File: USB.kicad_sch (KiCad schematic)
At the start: 15 parts, among them J2 USB4215-03-A, U8 CP2102N-A02-GQFN24

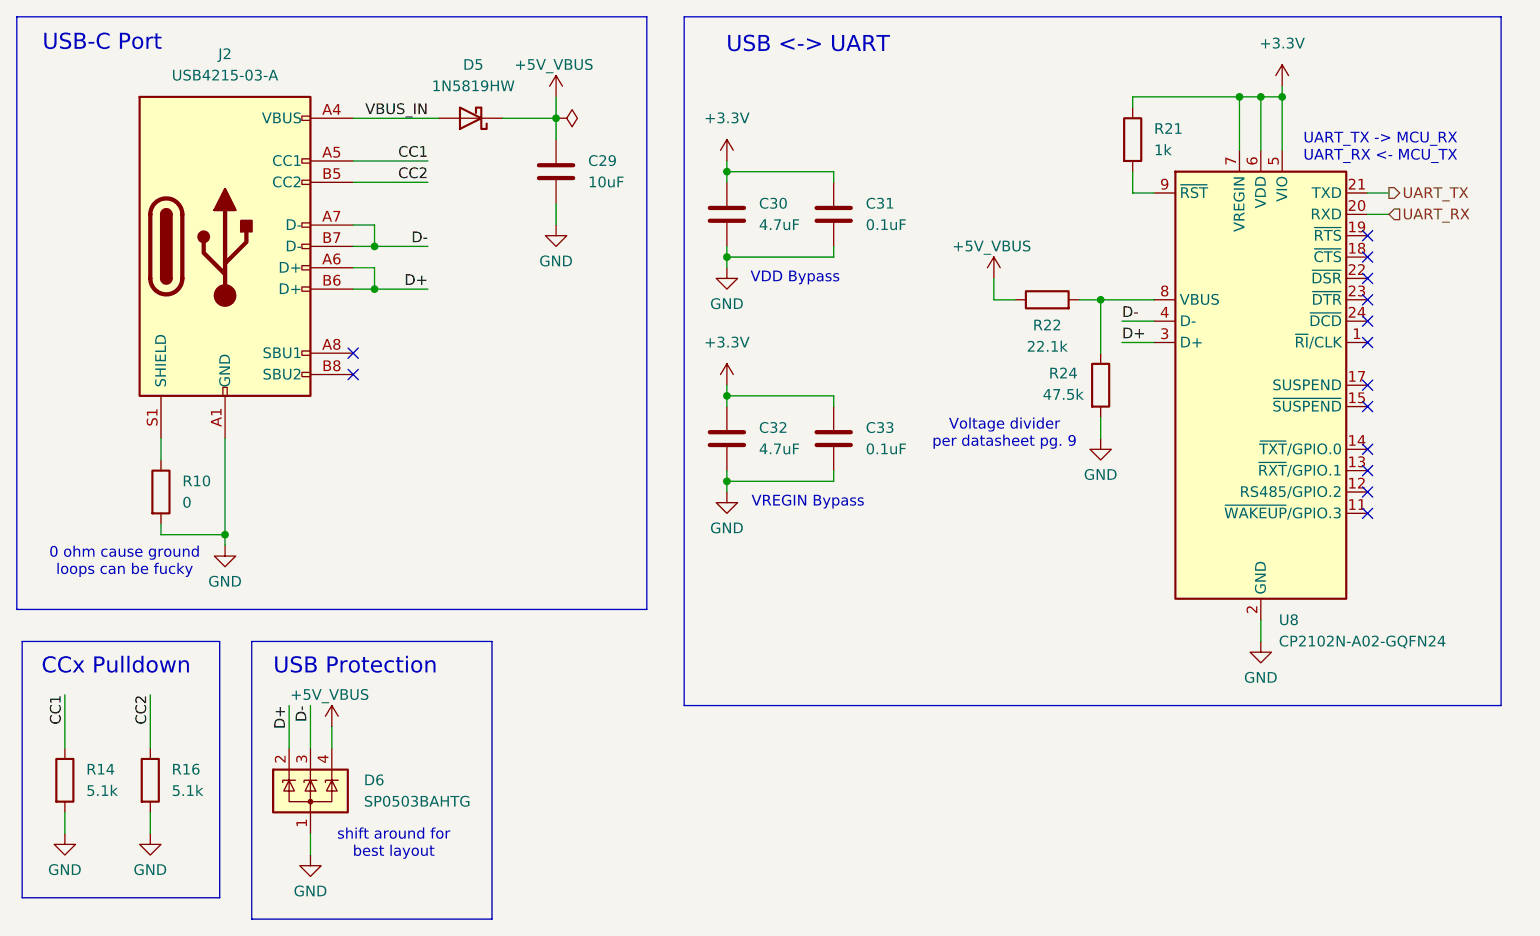
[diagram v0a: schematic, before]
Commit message: finish mcu breakouts
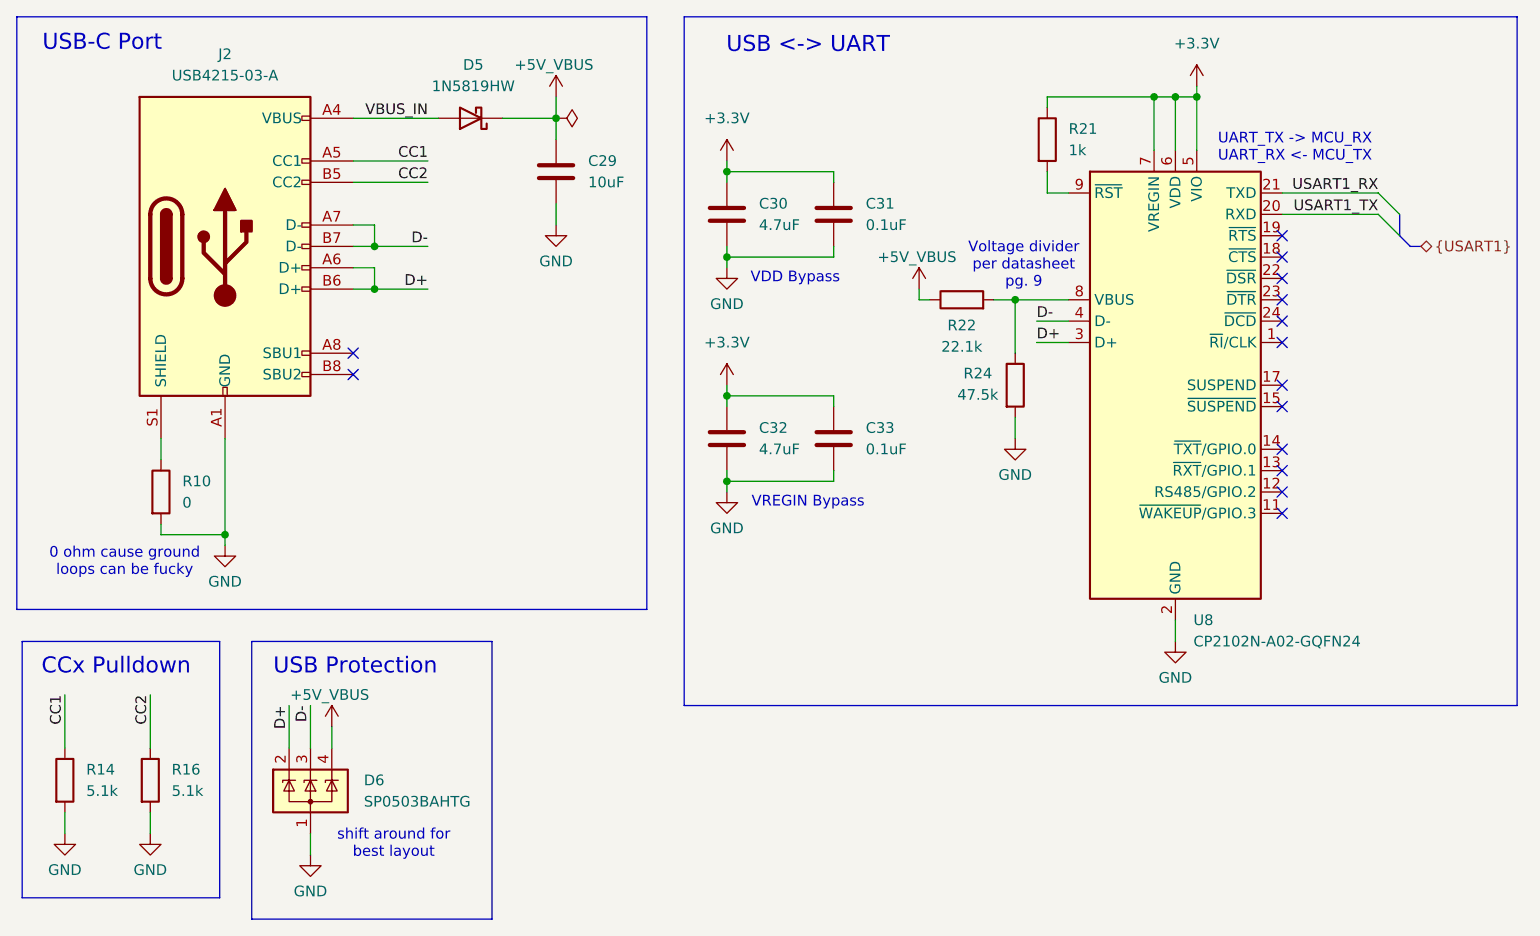
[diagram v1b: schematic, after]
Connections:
- net UART_RX renamed USART1_TX
- net UART_TX renamed USART1_RX
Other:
- moved on the sheet: R21, R22, R24, U8

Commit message: FUCK capacitors
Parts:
- C29: P/N (none) -> GRM21BR61H106KE43K
- C30, C32: P/N (none) -> 08055D475KAT4A
- C31, C33: P/N (none) -> MLASH168SB7104KTNA01
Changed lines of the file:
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@@
+			)
+		)
+		(property "P/N" "08055D475KAT4A"
+			(at 100.33 39.37 0)
+			(effects
+				(font
+					(size 1.27 1.27)
+				)
+				(hide yes)
 			)
 		)
@@
 			)
 		)
+		(property "P/N" "MLASH168SB7104KTNA01"
+			(at 113.03 66.04 0)
+			(effects
+				(font
+					(size 1.27 1.27)
+				)
+				(hide yes)
+			)
+		)
 		(pin "1"
 		)
@@
 			)
 		)
+		(property "P/N" "08055D475KAT4A"
+			(at 100.33 66.04 0)
+			(effects
+				(font
+					(size 1.27 1.27)
+				)
+				(hide yes)
+			)
+		)
 		(pin "1"
 		)
@@
 			)
 		)
+		(property "P/N" "MLASH168SB7104KTNA01"
+			(at 113.03 39.37 0)
+			(effects
+				(font
+					(size 1.27 1.27)
+				)
+				(hide yes)
+			)
+		)
 		(pin "1"
 		)
@@
 			(at 80.01 34.29 0)
 			(effects
+				(font
+					(size 1.27 1.27)
+				)
+				(hide yes)
+			)
+		)
+		(property "P/N" "GRM21BR61H106KE43K"
+			(at 80.01 34.29 0)
+			(effects

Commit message: all parts selected
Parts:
- R10: P/N (none) -> CRCW06030000Z0EI
- R14, R16: P/N (none) -> CRCW06035K10FKEC
- R21: P/N (none) -> CRCW06031K00FKEI
- R22: P/N (none) -> CRCW060322K1FKEBC
- R24: P/N (none) -> CRCW060347K5FKEAHP
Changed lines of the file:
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@@
+			)
+		)
+		(property "P/N" "CRCW06030000Z0EI "
+			(at 33.02 72.39 0)
+			(effects
+				(font
+					(size 1.27 1.27)
+				)
+				(hide yes)
 			)
 		)
@@
 		)
 		(property "Description" "Resistor"
+			(at 134.62 59.69 0)
+			(effects
+				(font
+					(size 1.27 1.27)
+				)
+				(hide yes)
+			)
+		)
+		(property "P/N" "CRCW060347K5FKEAHP "
 			(at 134.62 59.69 0)
 			(effects
@@
 			)
 		)
+		(property "P/N" "CRCW06035K10FKEC "
+			(at 31.75 106.68 0)
+			(effects
+				(font
+					(size 1.27 1.27)
+				)
+				(hide yes)
+			)
+		)
 		(pin "1"
 		)
@@
 		(property "Description" "Resistor"
 			(at 128.27 49.53 0)
+			(effects
+				(font
+					(size 1.27 1.27)
+				)
+				(hide yes)
+			)
+		)
+		(property "P/N" "CRCW060322K1FKEBC "
+			(at 128.27 49.53 90)
 			(effects
 				(font
@@
 			)
 		)
+		(property "P/N" "CRCW06031K00FKEI "
+			(at 138.43 30.48 0)
+			(effects
+				(font
+					(size 1.27 1.27)
+				)
+				(hide yes)
+			)
+		)
 		(pin "1"
 		)
@@
 			(at 21.59 106.68 0)
 			(effects
+				(font
+					(size 1.27 1.27)
+				)
+				(hide yes)
+			)
+		)
+		(property "P/N" "CRCW06035K10FKEC "
+			(at 21.59 106.68 0)
+			(effects

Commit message: add some footprints
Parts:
- R10, R14, R16, R21, R22, R24: footprint (none) -> Resistor_SMD:R_0603_1608Metric_Pad0.98x0.95mm_HandSolder
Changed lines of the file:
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@@
 			)
 		)
-		(property "Footprint" ""
+		(property "Footprint" "Resistor_SMD:R_0603_1608Metric_Pad0.98x0.95mm_HandSolder"
 			(at 31.242 72.39 90)
 			(effects
@@
 			)
 		)
-		(property "Footprint" ""
+		(property "Footprint" "Resistor_SMD:R_0603_1608Metric_Pad0.98x0.95mm_HandSolder"
 			(at 132.842 59.69 90)
 			(effects
@@
 			)
 		)
-		(property "Footprint" ""
+		(property "Footprint" "Resistor_SMD:R_0603_1608Metric_Pad0.98x0.95mm_HandSolder"
 			(at 29.972 106.68 90)
 			(effects
@@
 			)
 		)
-		(property "Footprint" ""
+		(property "Footprint" "Resistor_SMD:R_0603_1608Metric_Pad0.98x0.95mm_HandSolder"
 			(at 128.27 51.308 90)
 			(effects
@@
 			)
 		)
-		(property "Footprint" ""
+		(property "Footprint" "Resistor_SMD:R_0603_1608Metric_Pad0.98x0.95mm_HandSolder"
 			(at 136.652 30.48 90)
 			(effects
@@
 			)
 		)
-		(property "Footprint" ""
+		(property "Footprint" "Resistor_SMD:R_0603_1608Metric_Pad0.98x0.95mm_HandSolder"
 			(at 19.812 106.68 90)
 			(effects

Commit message: more stuff
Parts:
- J2: footprint (none) -> USB4215-03-A:GCT_USB4215-03-A_REVA
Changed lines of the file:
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@@
 			)
 		)
-		(property "Footprint" ""
+		(property "Footprint" "USB4215-03-A:GCT_USB4215-03-A_REVA"
 			(at 44.45 43.18 0)
 			(effects

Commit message: all footprints assigned
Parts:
- C29, C30, C32: footprint (none) -> Capacitor_SMD:C_0805_2012Metric_Pad1.18x1.45mm_HandSolder
- C31, C33: footprint (none) -> Capacitor_SMD:C_0603_1608Metric_Pad1.08x0.95mm_HandSolder
- D5: footprint (none) -> Diode_SMD:D_SOD-123
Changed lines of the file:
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@@
 			)
 		)
-		(property "Footprint" ""
+		(property "Footprint" "Diode_SMD:D_SOD-123"
 			(at 69.85 27.94 0)
 			(effects
@@
 			)
 		)
-		(property "Footprint" ""
+		(property "Footprint" "Capacitor_SMD:C_0805_2012Metric_Pad1.18x1.45mm_HandSolder"
 			(at 101.2952 43.18 0)
 			(effects
@@
 			)
 		)
-		(property "Footprint" ""
+		(property "Footprint" "Capacitor_SMD:C_0603_1608Metric_Pad1.08x0.95mm_HandSolder"
 			(at 113.9952 69.85 0)
 			(effects
@@
 			)
 		)
-		(property "Footprint" ""
+		(property "Footprint" "Capacitor_SMD:C_0805_2012Metric_Pad1.18x1.45mm_HandSolder"
 			(at 101.2952 69.85 0)
 			(effects
@@
 			)
 		)
-		(property "Footprint" ""
+		(property "Footprint" "Capacitor_SMD:C_0603_1608Metric_Pad1.08x0.95mm_HandSolder"
 			(at 113.9952 43.18 0)
 			(effects
@@
 			)
 		)
-		(property "Footprint" ""
+		(property "Footprint" "Capacitor_SMD:C_0805_2012Metric_Pad1.18x1.45mm_HandSolder"
 			(at 80.9752 38.1 0)
 			(effects
